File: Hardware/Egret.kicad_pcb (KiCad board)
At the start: 2 copper layers, 65 parts, among them J1 Conn_01x02_Male, J2 Conn_01x04_Male, J3 Conn_01x20_Male, J4 Conn_01x20_Male, Q1 AO3415AL, Q2 S8050, Q3 S8050, SW1 TD-1106SN-5.0H-160, SW2 TD-1106SN-5.0H-160, U1 WS2812B-B, U10 FPC-1.0FX-12PWBH20, U2 AN2051-245_2.4G, U3 BH1750FVI-TR, U4 ESP32--PICO--D4, U5 AMS1117-3.3, U6 FPC-1.0FX-12PWBH20, U7 CP2102-GMR-YJLTY, U8 MPU6050-YJLTY, U9 LP2992IM5-3.3

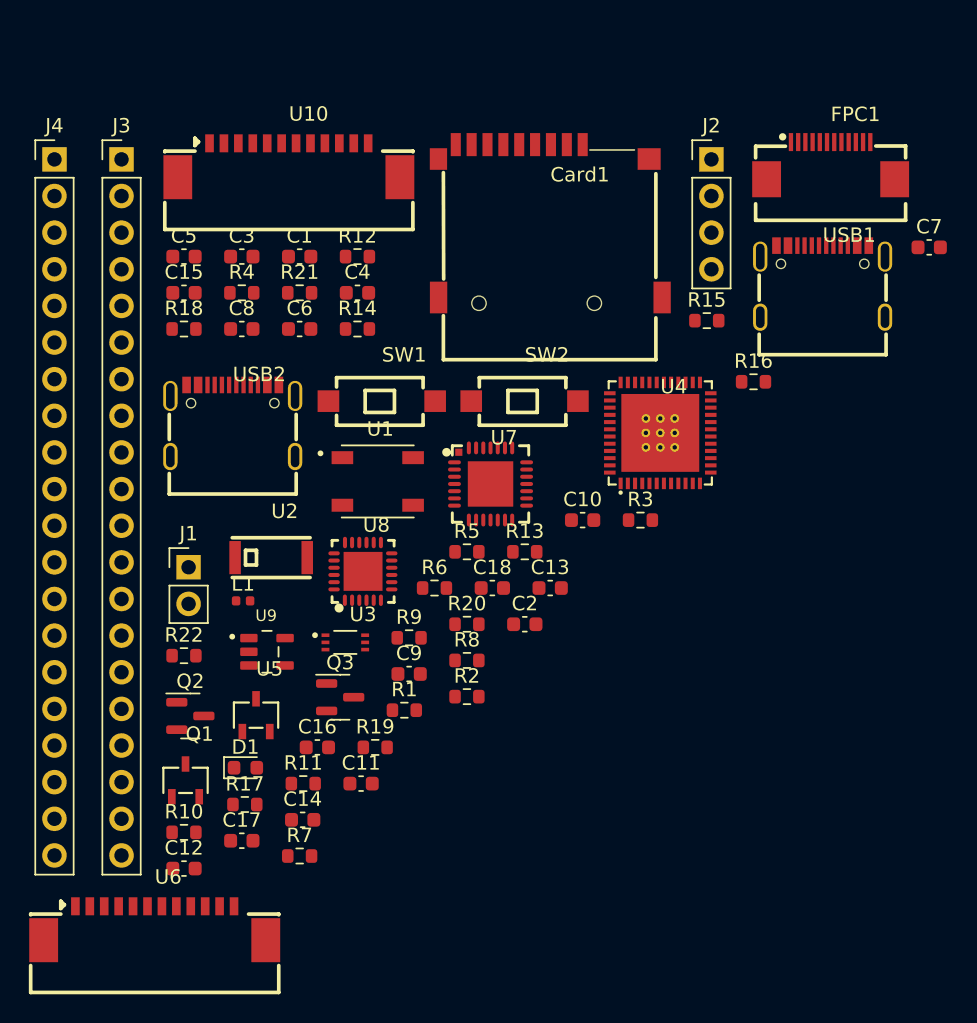
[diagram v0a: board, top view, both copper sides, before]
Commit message: update
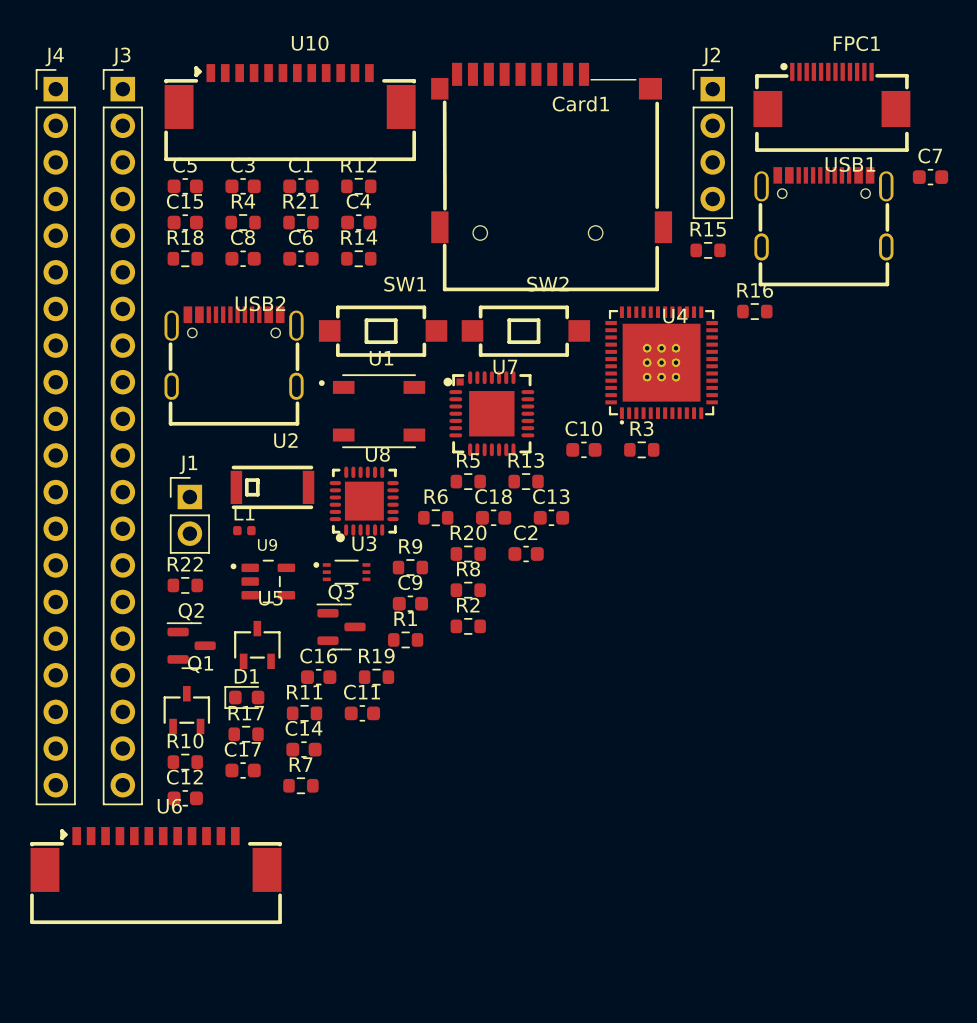
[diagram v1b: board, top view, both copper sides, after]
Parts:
- moved C1 4.87 mm to (138.9, 76.1)
- moved C10 4.87 mm to (158.5, 94.4)
- moved C14 4.87 mm to (139.1, 115.2)
- moved C17 4.87 mm to (134.9, 116.6)
- moved C2 4.87 mm to (154.5, 101.6)
- moved C3 4.87 mm to (134.9, 76.1)
- moved C6 4.87 mm to (138.9, 81.2)
- moved C7 4.87 mm to (182.6, 75.5)
- moved C8 4.87 mm to (134.9, 81.2)
- moved C9 4.87 mm to (146.5, 105.1)
- moved D1 4.87 mm to (135.2, 111.6)
- moved FPC1 4.87 mm to (175.7, 69.5)
- moved Q1 4.87 mm to (131.0, 112.5)
- moved Q2 4.87 mm to (131.3, 108.0)
- moved Q3 4.87 mm to (141.7, 106.7)
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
